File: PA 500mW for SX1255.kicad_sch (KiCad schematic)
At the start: 34 parts, among them J1 RF-in, J2 RF-out, J3 5Vcc input, U2 TQP7M9106

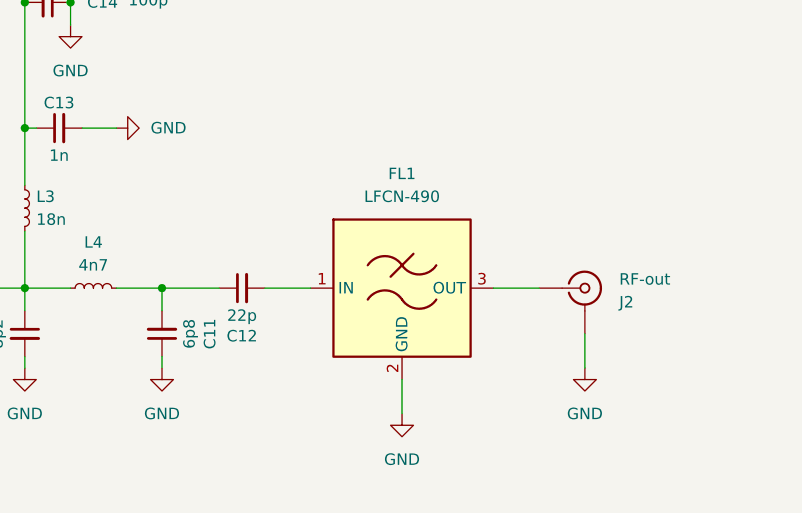
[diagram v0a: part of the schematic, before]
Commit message: Add files via upload
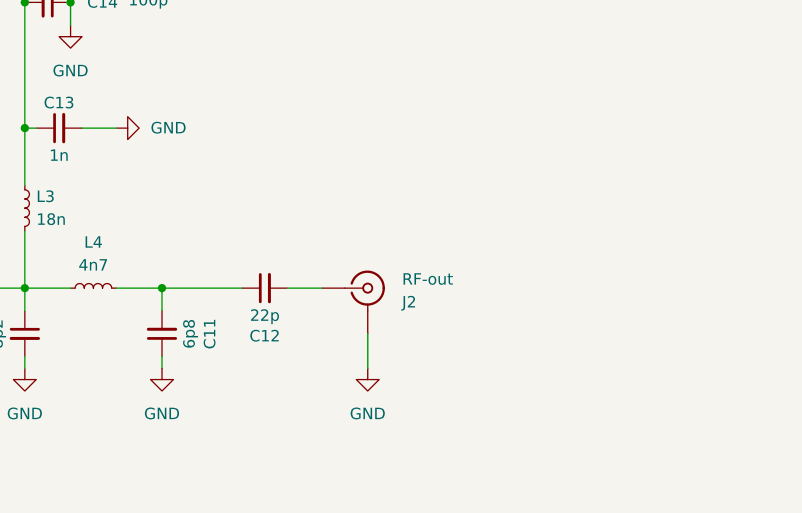
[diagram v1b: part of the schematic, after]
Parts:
- removed FL1: LFCN-490, Filter:Filter_Mini-Circuits_FV1206, symbol RF_Filter:LFCN-490
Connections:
- net at C12.2: now also J2.1 (In)
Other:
- moved on the sheet: C12, J2
